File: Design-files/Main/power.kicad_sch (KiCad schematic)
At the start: 24 parts, among them J2 Battery Jumper, J8 Conn_01x04_Pin, U4 LTC4054ES5-4.2, U6 TPS2115A-Q1, U7 RT9073A

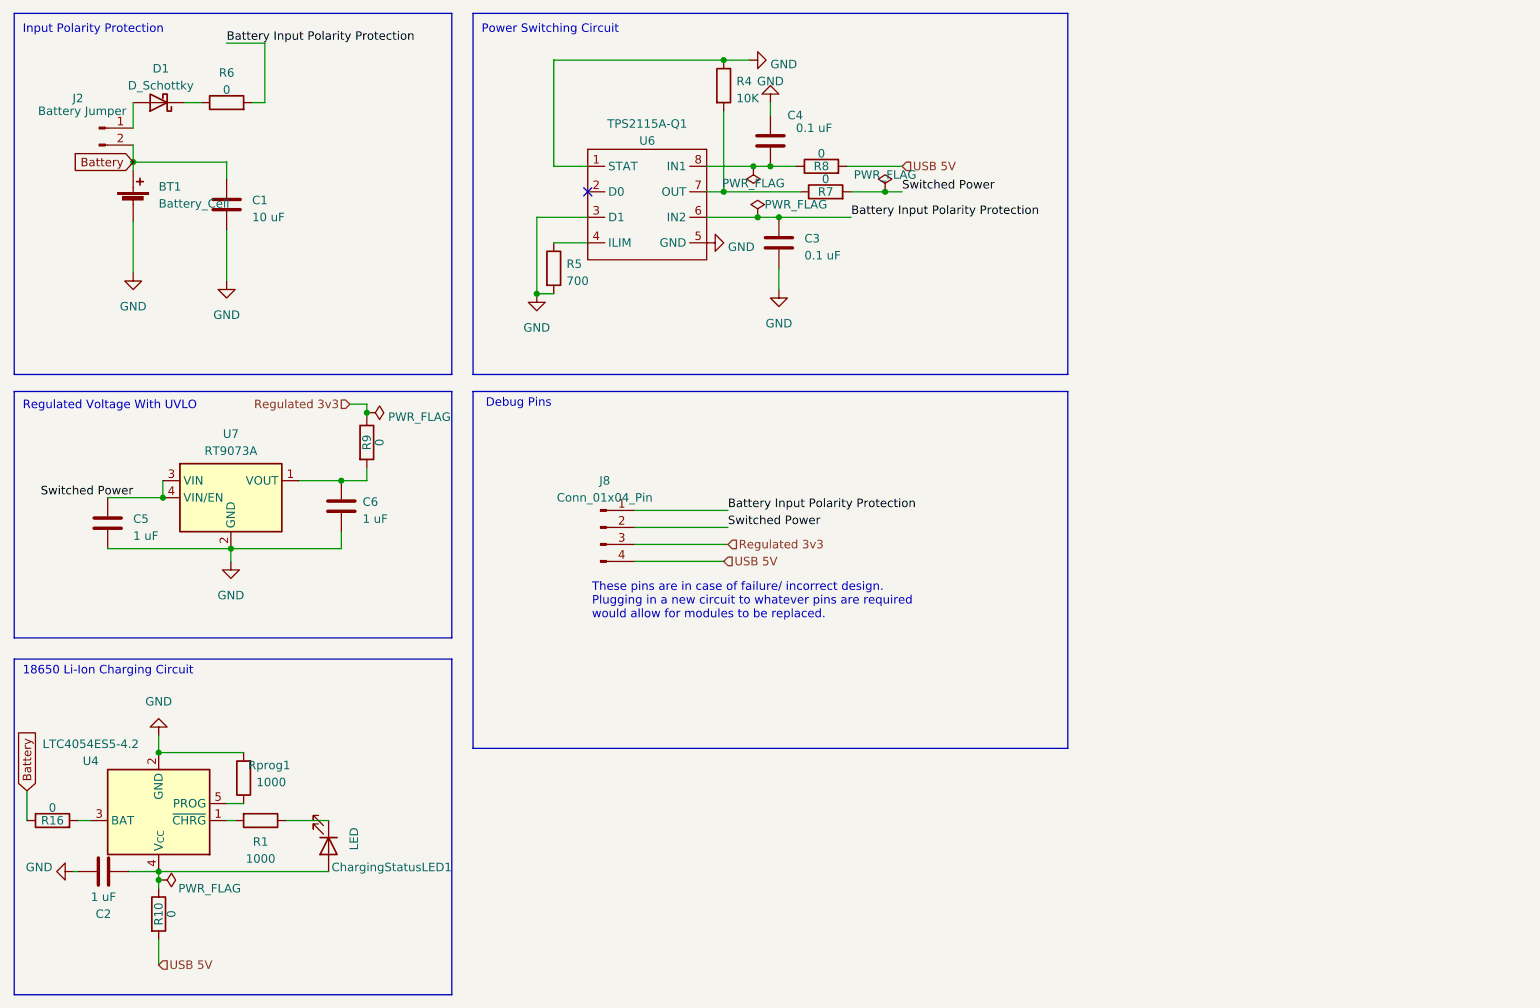
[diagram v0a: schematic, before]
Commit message: lets go team
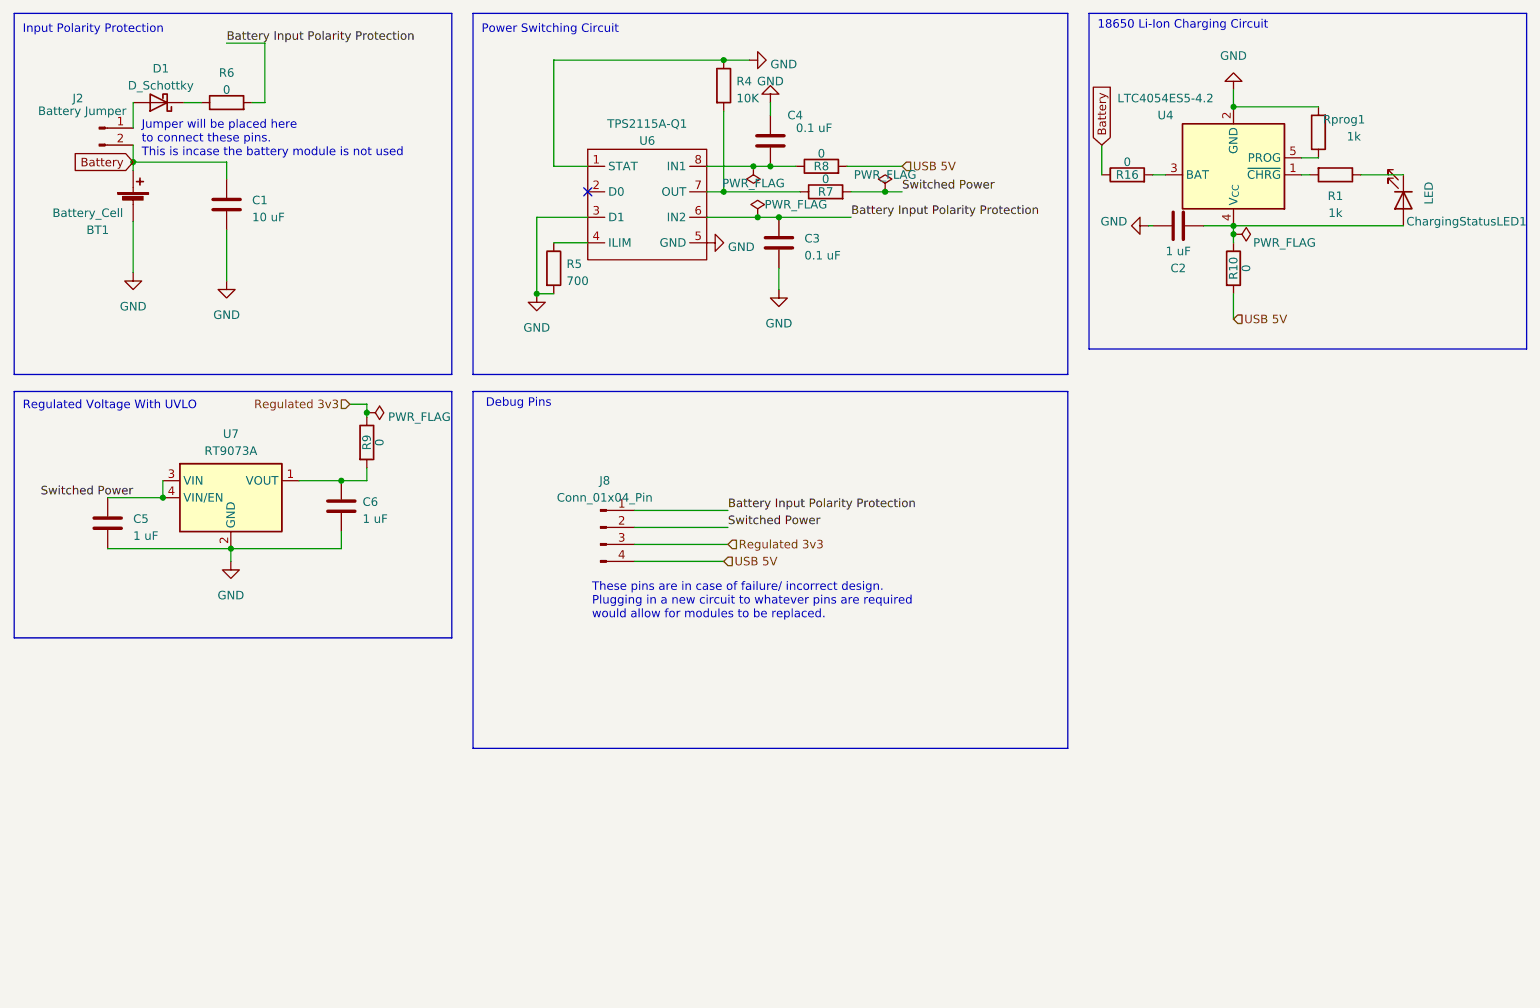
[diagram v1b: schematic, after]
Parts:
- R1, Rprog1: value 1000 -> 1k
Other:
- note added: "Jumper will be placed here to connect these pins. This is incase the battery module is not used"
- moved on the sheet: C2, ChargingStatusLED1, R1, R10, R16, Rprog1, U4
